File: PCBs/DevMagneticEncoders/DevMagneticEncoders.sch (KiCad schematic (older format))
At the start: 23 parts, among them J1 Conn_01x06_Male, J2 Conn_01x06_Male, J3 Screw_Terminal_01x02, J4 Conn_02x03_Odd_Even, J5 Conn_02x03_Odd_Even, J6 Conn_01x06_Male, J7 Conn_01x04_Male, J8 Conn_01x04_Male, U1 AZ1117-3.3, U2 ESP32-S2-WROOM

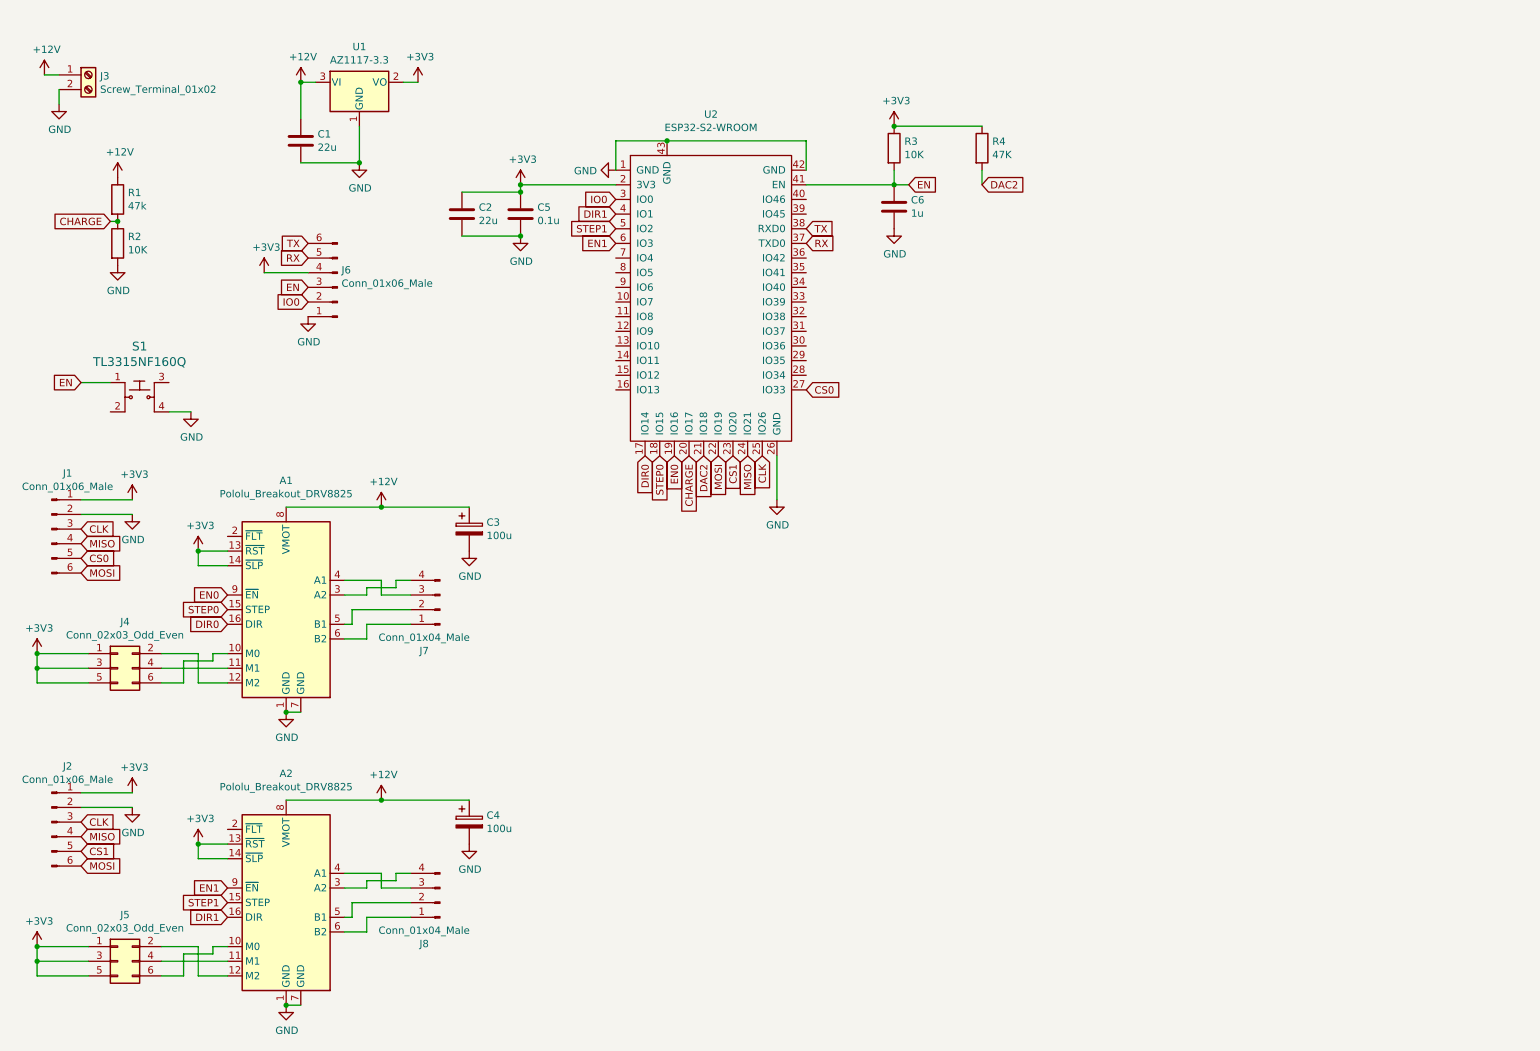
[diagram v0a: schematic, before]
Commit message: 5 stepper board
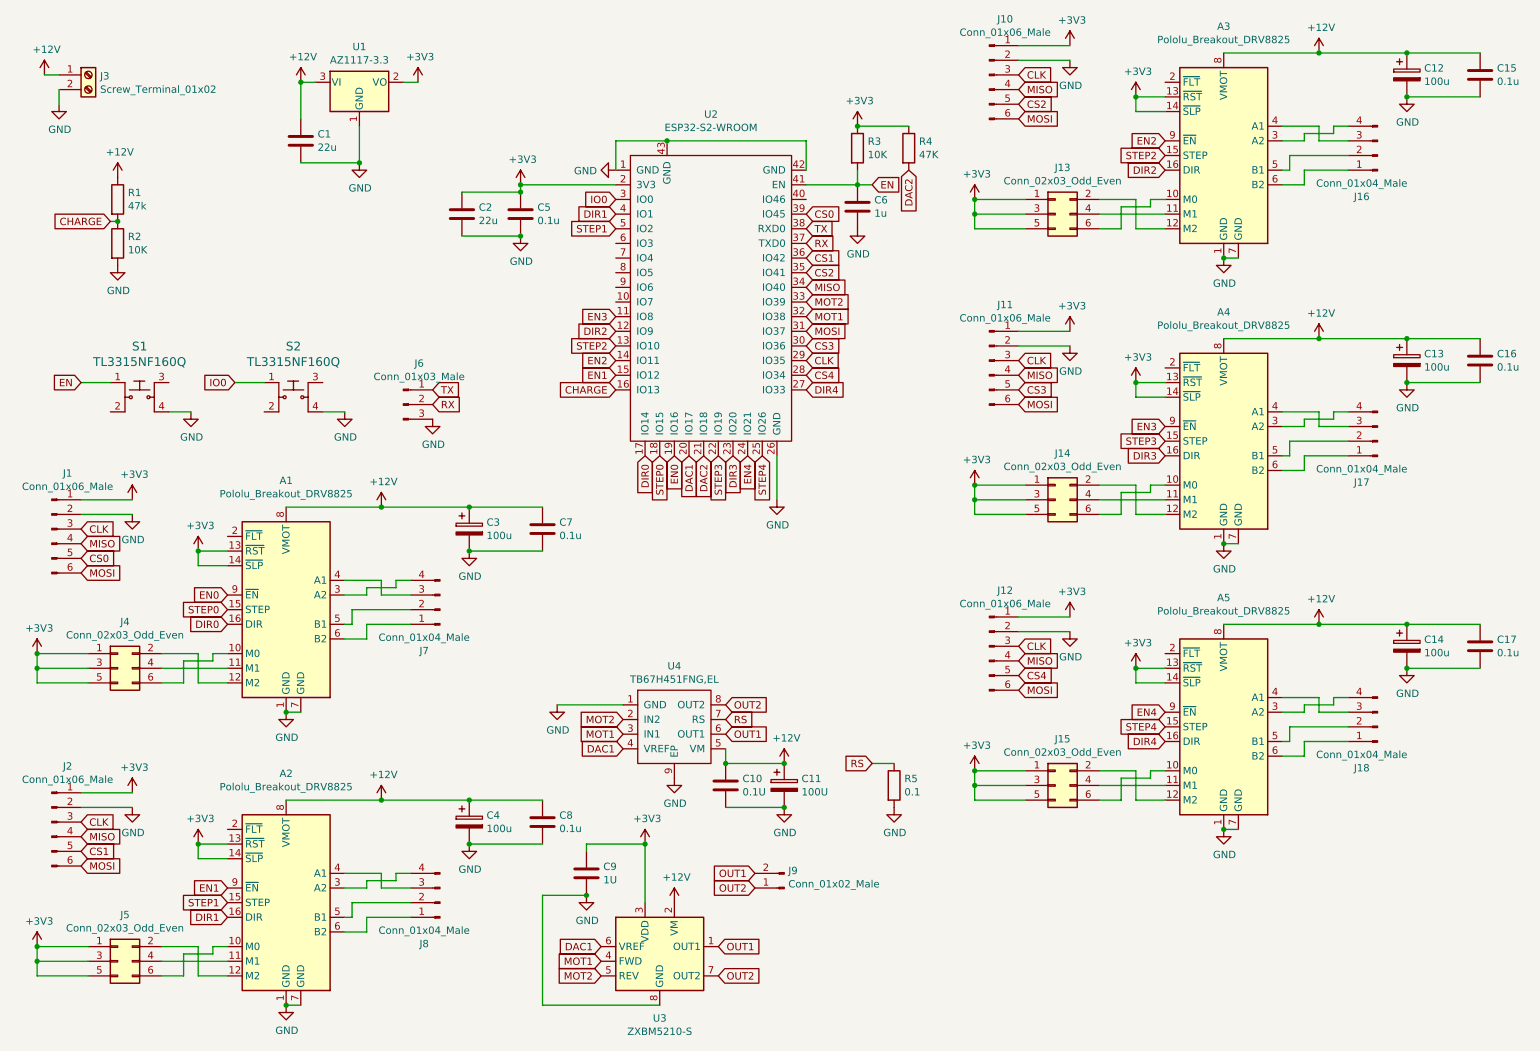
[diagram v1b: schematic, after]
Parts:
- removed J6: Conn_01x06_Male, Connector_JST:JST_PH_B6B-PH-K_1x06_P2.00mm_Vertical, symbol Connector:Conn_01x06_Male
- added A3, A4, A5: Pololu_Breakout_DRV8825, Module:Pololu_Breakout-16_15.2x20.3mm, symbol Driver_Motor:Pololu_Breakout_DRV8825
- added C10: 0.1U, Capacitor_SMD:C_0805_2012Metric_Pad1.18x1.45mm_HandSolder, symbol Device:C
- added C11: 100U, Capacitor_SMD:CP_Elec_6.3x7.7, symbol Device:CP
- added C12, C13, C14: 100u, Capacitor_SMD:CP_Elec_6.3x7.7, symbol Device:CP
- added C15, C16, C17, C7, C8: 0.1u, Capacitor_SMD:C_0805_2012Metric_Pad1.18x1.45mm_HandSolder, symbol Device:C
- added C9: 1U, Capacitor_SMD:C_0805_2012Metric_Pad1.18x1.45mm_HandSolder, symbol Device:C
- added J10, J11, J12: Conn_01x06_Male, Connector_JST:JST_XH_B6B-XH-A_1x06_P2.50mm_Vertical, symbol Connector:Conn_01x06_Male
- added J13, J14, J15: Conn_02x03_Odd_Even, Connector_PinHeader_2.54mm:PinHeader_2x03_P2.54mm_Vertical, symbol Connector_Generic:Conn_02x03_Odd_Even
- added J16, J17, J18: Conn_01x04_Male, Connector_JST:JST_XH_B4B-XH-A_1x04_P2.50mm_Vertical, symbol Connector:Conn_01x04_Male
- added J6: Conn_01x03_Male, Connector_PinHeader_2.54mm:PinHeader_1x03_P2.54mm_Vertical, symbol Connector:Conn_01x03_Male
- added J9: Conn_01x02_Male, Connector_JST:JST_XH_B2B-XH-A_1x02_P2.50mm_Vertical, symbol Connector:Conn_01x02_Male
- added R5: 0.1, Resistor_SMD:R_0805_2012Metric_Pad1.20x1.40mm_HandSolder, symbol Device:R
- added S2: TL3315NF160Q, A4:TL3305AF160QG, symbol dk_Tactile-Switches:TL3315NF160Q
- added U3: ZXBM5210-S, Package_SO:SOIC-8_3.9x4.9mm_P1.27mm, symbol Driver_Motor:ZXBM5210-S
- added U4: TB67H451FNG,EL, Package_SO:SOIC-8-1EP_3.9x4.9mm_P1.27mm_EP2.29x3mm_ThermalVias, symbol BoilerBot:TB67H451FNG,EL
- S1: footprint A4:CK_PTS647_4.5x4.5 -> A4:TL3305AF160QG
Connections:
- net +12V: now also A3.8 (VMOT), A4.8 (VMOT), A5.8 (VMOT), C10.1, C11.1, C12.1, C13.1, C14.1, C15.1, C16.1, C17.1, C7.1, C8.1, U3.2 (VM), U4.5 (VM)
- net +3V3: now also A3.13 (~RST), A3.14 (~SLP), A4.13 (~RST), A4.14 (~SLP), A5.13 (~RST), A5.14 (~SLP), C9.1, J10.1 (Pin_1), J11.1 (Pin_1), J12.1 (Pin_1), J13.1 (Pin_1), J13.3 (Pin_3), J13.5 (Pin_5), J14.1 (Pin_1), J14.3 (Pin_3), J14.5 (Pin_5), J15.1 (Pin_1), J15.3 (Pin_3), J15.5 (Pin_5), U3.3 (VDD)
- net CHARGE: now also U2.16 (IO13); no longer U2.20 (IO17)
- net CLK: now also U2.29 (IO35), J10.3 (Pin_3), J11.3 (Pin_3), J12.3 (Pin_3); no longer U2.25 (IO26)
- net CS0: now also U2.39 (IO45); no longer U2.27 (IO33)
- net CS1: now also U2.36 (IO42); no longer U2.23 (IO20)
- net EN1: now also U2.15 (IO12); no longer U2.6 (IO3)
- net GND: now also A3.1 (GND), A3.7 (GND), A4.1 (GND), A4.7 (GND), A5.1 (GND), A5.7 (GND), C10.2, C11.2, C12.2, C13.2, C14.2, C15.2, C16.2, C17.2, C7.2, C8.2, C9.2, J10.2 (Pin_2), J11.2 (Pin_2), J12.2 (Pin_2), J6.3 (Pin_3), R5.2, S2.4, U3.8 (GND), U4.1 (GND), U4.9 (EP)
- net IO0: now also S2.1
- net MISO: now also U2.34 (IO40), J10.4 (Pin_4), J11.4 (Pin_4), J12.4 (Pin_4); no longer U2.24 (IO21)
- net MOSI: now also U2.31 (IO37), J10.6 (Pin_6), J11.6 (Pin_6), J12.6 (Pin_6); no longer U2.22 (IO19)
- net RX: now also J6.2 (Pin_2)
- net TX: now also J6.1 (Pin_1)
- net EN3: now reaches U2.11 (IO8)
- net EN3: now also A4.9 (~EN)
- net DIR2: now reaches U2.12 (IO9)
- net DIR2: now also A3.16 (DIR)
- net STEP2: now reaches U2.13 (IO10)
- net STEP2: now also A3.15 (STEP)
- net EN2: now reaches U2.14 (IO11)
- net EN2: now also A3.9 (~EN)
- net CS4: now reaches U2.28 (IO34)
- net CS4: now also J12.5 (Pin_5)
- net CS3: now reaches U2.30 (IO36)
- net CS3: now also J11.5 (Pin_5)
- net MOT1: now reaches U2.32 (IO38)
- net MOT1: now also U3.4 (FWD), U4.3 (IN1)
- net MOT2: now reaches U2.33 (IO39)
- net MOT2: now also U3.5 (REV), U4.2 (IN2)
- net CS2: now reaches U2.35 (IO41)
- net CS2: now also J10.5 (Pin_5)
- new net: A5.12 (M2), J15.2 (Pin_2)
- new net: A5.11 (M1), J15.4 (Pin_4)
- new net: A5.10 (M0), J15.6 (Pin_6)
- new net: A5.6 (B2), J18.1 (Pin_1)
- new net: A5.5 (B1), J18.2 (Pin_2)
- new net: A5.4 (A1), J18.3 (Pin_3)
- new net: A5.3 (A2), J18.4 (Pin_4)
- new net: A4.12 (M2), J14.2 (Pin_2)
- new net: A4.11 (M1), J14.4 (Pin_4)
- new net: A4.10 (M0), J14.6 (Pin_6)
- new net: A4.6 (B2), J17.1 (Pin_1)
- new net: A4.5 (B1), J17.2 (Pin_2)
- new net: A4.4 (A1), J17.3 (Pin_3)
- new net: A4.3 (A2), J17.4 (Pin_4)
- new net: A3.12 (M2), J13.2 (Pin_2)
- new net: A3.11 (M1), J13.4 (Pin_4)
- new net: A3.10 (M0), J13.6 (Pin_6)
- new net: A3.6 (B2), J16.1 (Pin_1)
- new net: A3.5 (B1), J16.2 (Pin_2)
- new net: A3.4 (A1), J16.3 (Pin_3)
- new net: A3.3 (A2), J16.4 (Pin_4)
- new net DAC1: U2.20 (IO17), U3.6 (VREF), U4.4 (VREF)
- new net DIR3: A4.16 (DIR), U2.23 (IO20)
- new net DIR4: A5.16 (DIR), U2.27 (IO33)
- new net EN4: A5.9 (~EN), U2.24 (IO21)
- new net OUT1: J9.2 (Pin_2), U3.1 (OUT1), U4.6 (OUT1)
- new net OUT2: J9.1 (Pin_1), U3.7 (OUT2), U4.8 (OUT2)
- new net RS: R5.1, U4.7 (RS)
- new net STEP3: A4.15 (STEP), U2.22 (IO19)
- new net STEP4: A5.15 (STEP), U2.25 (IO26)
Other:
- moved on the sheet: C6, R3, R4
